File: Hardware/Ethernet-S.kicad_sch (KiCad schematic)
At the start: 15 parts, among them J1 Conn_01x07_Male, J10 SPI, J11 Conn_01x10_Male, J12 Conn_01x04_Male, J2 Conn_01x04_Male, J3 Conn_01x02_Male, J4 Conn_01x02_Male, J5 Conn_01x02_Male, J6 Conn_01x02_Male, J7 Conn_01x08_Male, J8 SPI, J9 QWIIC_Stackable

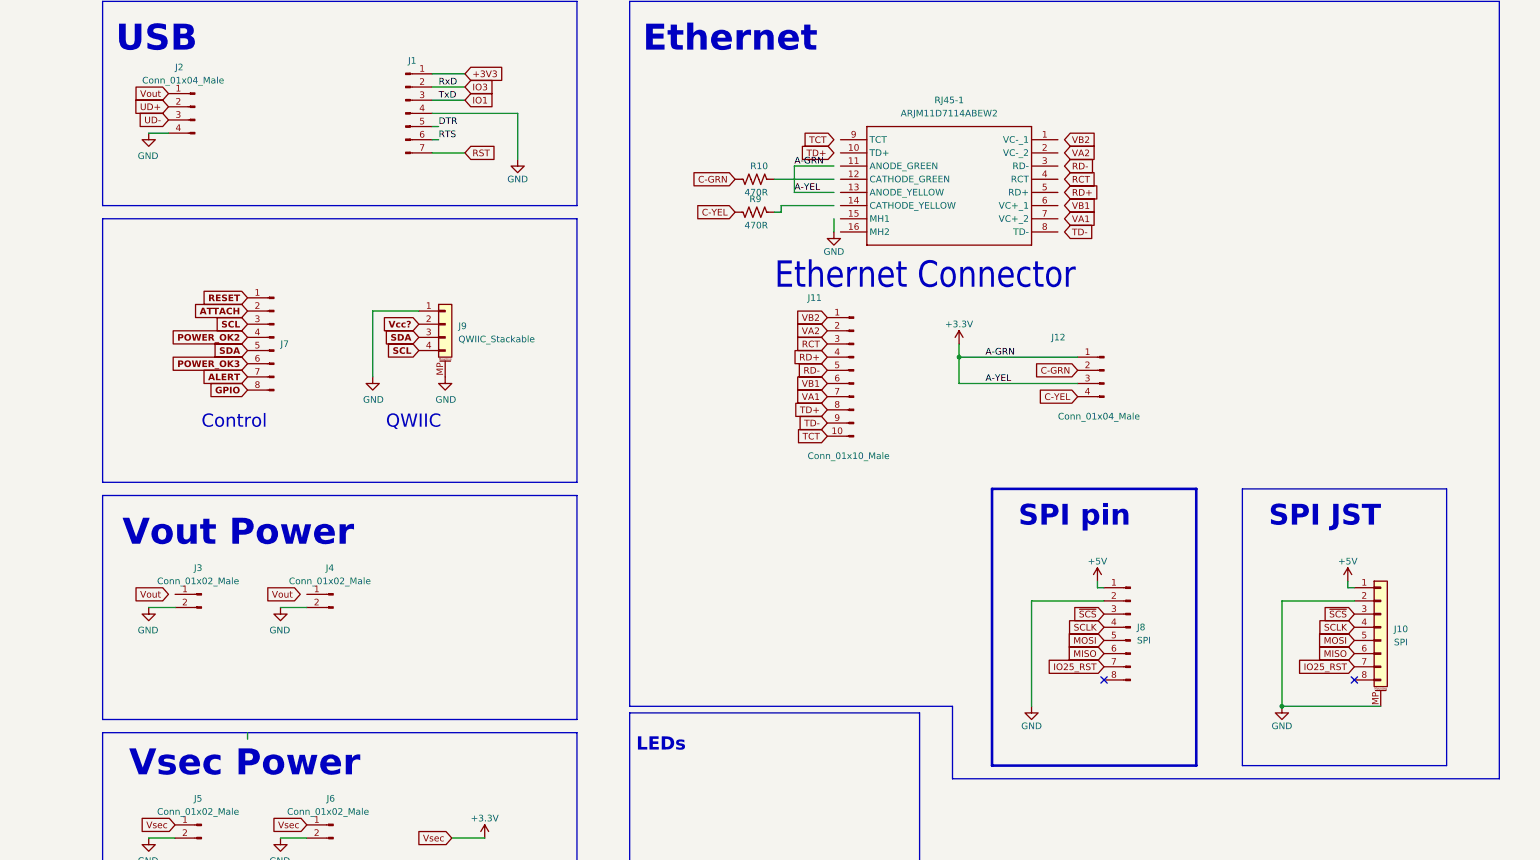
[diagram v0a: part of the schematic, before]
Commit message: Buncha cosmetic stuff...
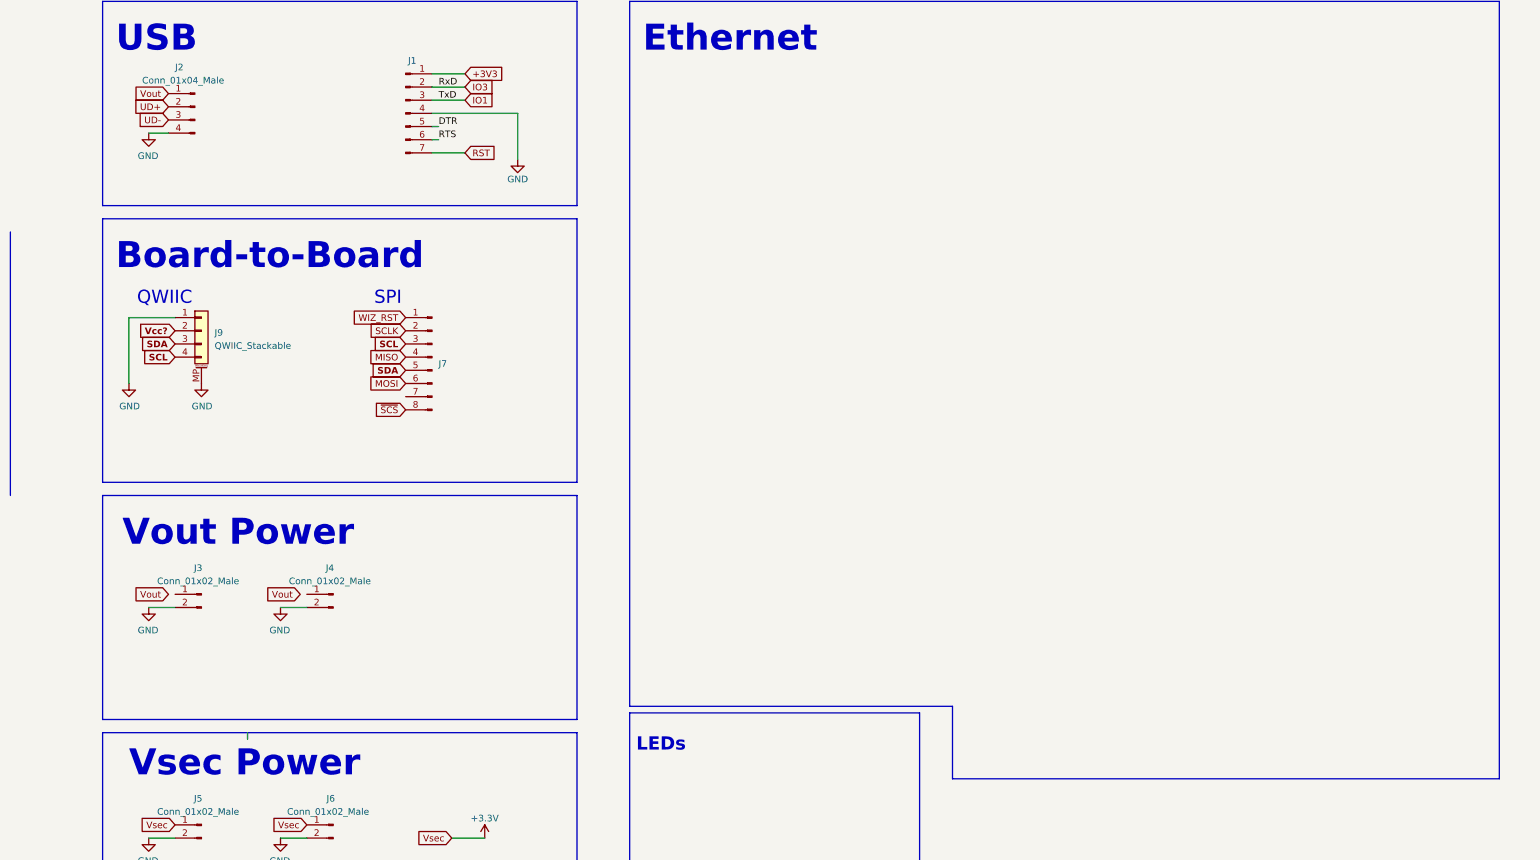
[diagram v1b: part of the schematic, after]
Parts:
- removed J10: SPI, bare-footprints:8 pin jst 1.25 vertical, symbol Connector_Generic_MountingPin:Conn_01x08_MountingPin
- removed J11: Conn_01x10_Male, Tinker:PinHeader_1x10_P1.27mm_Vertical, symbol Connector:Conn_01x10_Male
- removed J12: Conn_01x04_Male, Tinker:PinHeader_1x04_P1.27mm_Vertical, symbol Connector:Conn_01x04_Male
- removed J8: SPI, Tinker:PinHeader_1x08_P1.27mm_Vertical, symbol Connector:Conn_01x08_Male
- removed R10, R9: 470R, Resistor_SMD:R_0603_1608Metric, symbol Device:R_US
- removed RJ45-1: ARJM11D7114ABEW2, Tinker:CONN_ARJM11D7-114-AB-EW2_ABR, symbol ARJM11D7-114-AB-EW2_ABR:ARJM11D7114ABEW2
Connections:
- net ATTACH is gone; now on net SCLK: J7.2 (Pin_2)
- net GPIO is gone; now on net ~{SCS}: J7.8 (Pin_8)
- net POWER_OK2 is gone; now on net MISO: J7.4 (Pin_4)
- net POWER_OK3 is gone; now on net MOSI: J7.6 (Pin_6)
- net ALERT: no longer names the net of J7.7 (Pin_7)
- net RESET renamed WIZ_RST
- no-connect marks 2 -> 0
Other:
- note added: "Board-to-Board"
- note added: "SPI"
- note removed: "Control"
- note removed: "Ethernet Connector"
- note removed: "SPI JST"
- note removed: "SPI pin"
- moved on the sheet: J7, J9
